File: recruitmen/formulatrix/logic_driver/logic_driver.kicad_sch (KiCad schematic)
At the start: 16 parts, among them J1 Sensor Input, J2 Sensor Input, J3 Motor Output, J4 Conn_01x02_Socket, J5 Conn_01x02_Socket, Q1 IRG4PF50W, U1 LM358_DFN, U2 4070, U3 4N35, U4 L7805

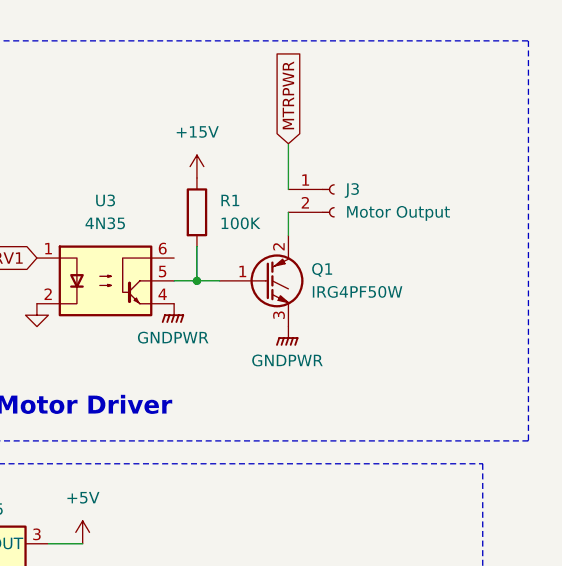
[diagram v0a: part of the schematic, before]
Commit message: PCB Recruitment
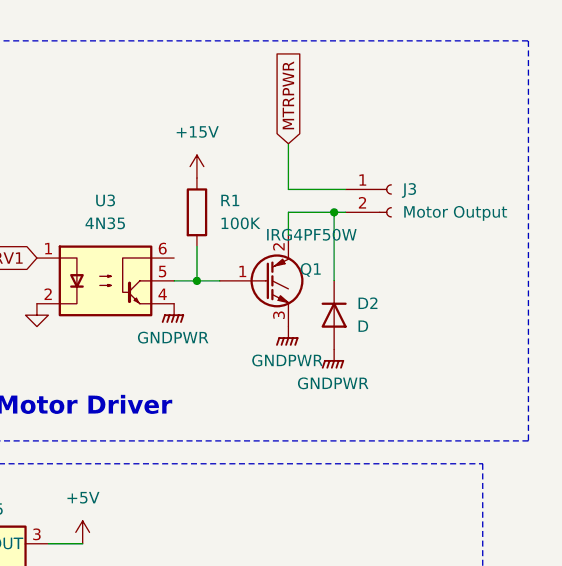
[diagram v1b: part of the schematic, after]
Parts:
- added D2: D, Diode_THT:D_A-405_P7.62mm_Horizontal, symbol Device:D
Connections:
- net GNDPWR: now also D2.2 (A)
- net at J3.2 (Pin_2), Q1.2 (C): now also D2.1 (K)
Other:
- moved on the sheet: J3
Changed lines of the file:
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@@
   (junction (at 153.67 74.93) (diameter 0) (color 0 0 0 0)
+  )
+  (junction (at 204.47 38.1) (diameter 0) (color 0 0 0 0)
   )
   (junction (at 58.42 34.29) (diameter 0) (color 0 0 0 0)
@@
     (stroke (width 0) (type default))
   )
+  (wire (pts (xy 199.39 30.48) (xy 199.39 35.56))
+    (stroke (width 0) (type default))
+  )
   (wire (pts (xy 81.28 46.99) (xy 81.28 49.53))
     (stroke (width 0) (type default))
@@
     (stroke (width 0) (type default))
   )
+  (wire (pts (xy 199.39 38.1) (xy 199.39 40.64))
+    (stroke (width 0) (type default))
+  )
   (wire (pts (xy 186.69 45.72) (xy 189.23 45.72))
     (stroke (width 0) (type default))
@@
     (stroke (width 0) (type default))
   )
-  (wire (pts (xy 199.39 38.1) (xy 199.39 40.64))
-    (stroke (width 0) (type default))
-  )
   (wire (pts (xy 148.59 74.93) (xy 153.67 74.93))
     (stroke (width 0) (type default))
   )
+  (wire (pts (xy 199.39 35.56) (xy 205.74 35.56))
+    (stroke (width 0) (type default))
+  )
   (wire (pts (xy 60.96 39.37) (xy 58.42 39.37))
     (stroke (width 0) (type default))
@@
     (stroke (width 0) (type default))
   )
+  (wire (pts (xy 204.47 38.1) (xy 204.47 45.72))
+    (stroke (width 0) (type default))
+  )
   (wire (pts (xy 172.72 74.93) (xy 176.53 74.93))
     (stroke (width 0) (type default))
@@
     (stroke (width 0) (type default))
   )
-  (wire (pts (xy 199.39 30.48) (xy 199.39 35.56))
+  (wire (pts (xy 205.74 38.1) (xy 204.47 38.1))
+    (stroke (width 0) (type default))
+  )
+  (wire (pts (xy 204.47 38.1) (xy 199.39 38.1))
     (stroke (width 0) (type default))
   )
@@
     )
   )
-  (symbol (lib_id "Connector:Conn_01x02_Socket") (at 204.47 35.56 0) (unit 1)
-    (in_bom yes) (on_board yes) (dnp no) (fields_autoplaced)
-    (property "Reference" "J3" (at 205.74 35.56 0)
-      (effects (font (size 1.27 1.27)) (justify left))
-    )
-    (property "Value" "Motor Output" (at 205.74 38.1 0)
-      (effects (font (size 1.27 1.27)) (justify left))
-    )
-    (property "Footprint" "TerminalBlock:TerminalBlock_Altech_AK300-2_P5.00mm" (at 204.47 35.56 0)
-      (effects (font (size 1.27 1.27)) hide)
-    )
-    (property "Datasheet" "~" (at 204.47 35.56 0)
+  (symbol (lib_id "Connector:Conn_01x02_Socket") (at 210.82 35.56 0) (unit 1)
+    (in_bom yes) (on_board yes) (dnp no) (fields_autoplaced)
+    (property "Reference" "J3" (at 212.09 35.56 0)
+      (effects (font (size 1.27 1.27)) (justify left))
+    )
+    (property "Value" "Motor Output" (at 212.09 38.1 0)
+      (effects (font (size 1.27 1.27)) (justify left))
+    )
+    (property "Footprint" "TerminalBlock:TerminalBlock_Altech_AK300-2_P5.00mm" (at 210.82 35.56 0)
+      (effects (font (size 1.27 1.27)) hide)
+    )
+    (property "Datasheet" "~" (at 210.82 35.56 0)
       (effects (font (size 1.27 1.27)) hide)
     )
@@
   )
   (symbol (lib_id "Transistor_IGBT:IRG4PF50W") (at 196.85 45.72 0) (unit 1)
-    (in_bom yes) (on_board yes) (dnp no) (fields_autoplaced)
-    (property "Reference" "Q1" (at 201.93 44.45 0)
-      (effects (font (size 1.27 1.27)) (justify left))
-    )
-    (property "Value" "IRG4PF50W" (at 201.93 46.99 0)
+    (in_bom yes) (on_board yes) (dnp no)
+    (property "Reference" "Q1" (at 200.66 44.45 0)
+      (effects (font (size 1.27 1.27)) (justify left))
+    )
+    (property "Value" "IRG4PF50W" (at 196.85 40.64 0)
       (effects (font (size 1.27 1.27)) (justify left))
     )
@@
         (path "/262f7926-104b-447c-8b8c-755c607a4b20"
           (reference "Q1") (unit 1)
+        )
+      )
+    )
+  )
+  (symbol (lib_id "power:GNDPWR") (at 204.47 53.34 0) (unit 1)
+    (in_bom yes) (on_board yes) (dnp no) (fields_autoplaced)
+    (property "Reference" "#PWR021" (at 204.47 58.42 0)
+      (effects (font (size 1.27 1.27)) hide)
+    )
+    (property "Value" "GNDPWR" (at 204.343 57.15 0)
+      (effects (font (size 1.27 1.27)))
+    )
+    (property "Footprint" "" (at 204.47 54.61 0)
+      (effects (font (size 1.27 1.27)) hide)
+    )
+    (property "Datasheet" "" (at 204.47 54.61 0)
+      (effects (font (size 1.27 1.27)) hide)
+    )
+    (pin "1")
+    (instances
+      (project "logic_driver"
+        (path "/262f7926-104b-447c-8b8c-755c607a4b20"
+          (reference "#PWR021") (unit 1)
         )
       )
@@
         )
       )
+    )
+  )
+  (symbol (lib_id "Device:D") (at 204.47 49.53 270) (unit 1)
+    (in_bom yes) (on_board yes) (dnp no) (fields_autoplaced)
+    (property "Reference" "D2" (at 207.01 48.26 90)
+      (effects (font (size 1.27 1.27)) (justify left))
+    )
+    (property "Value" "D" (at 207.01 50.8 90)
+      (effects (font (size 1.27 1.27)) (justify left))
+    )
+    (property "Footprint" "Diode_THT:D_A-405_P7.62mm_Horizontal" (at 204.47 49.53 0)
+      (effects (font (size 1.27 1.27)) hide)
+    )
+    (property "Datasheet" "~" (at 204.47 49.53 0)
+      (effects (font (size 1.27 1.27)) hide)
+    )
+    (property "Sim.Device" "D" (at 204.47 49.53 0)
+      (effects (font (size 1.27 1.27)) hide)
+    )
+    (property "Sim.Pins" "1=K 2=A" (at 204.47 49.53 0)
+      (effects (font (size 1.27 1.27)) hide)
+    )
+    (pin "1")
+    (pin "2")
+    (instances
+      (project "logic_driver"
+        (path "/262f7926-104b-447c-8b8c-755c607a4b20"
+          (reference "D2") (unit 1)
+        )
+      )
